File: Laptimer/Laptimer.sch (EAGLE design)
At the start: 64 parts, among them IC1 MCP73831/OT, IC5 NE555D, Q1 8mhz, Q4 PBSS4120T, X1 mini-usb

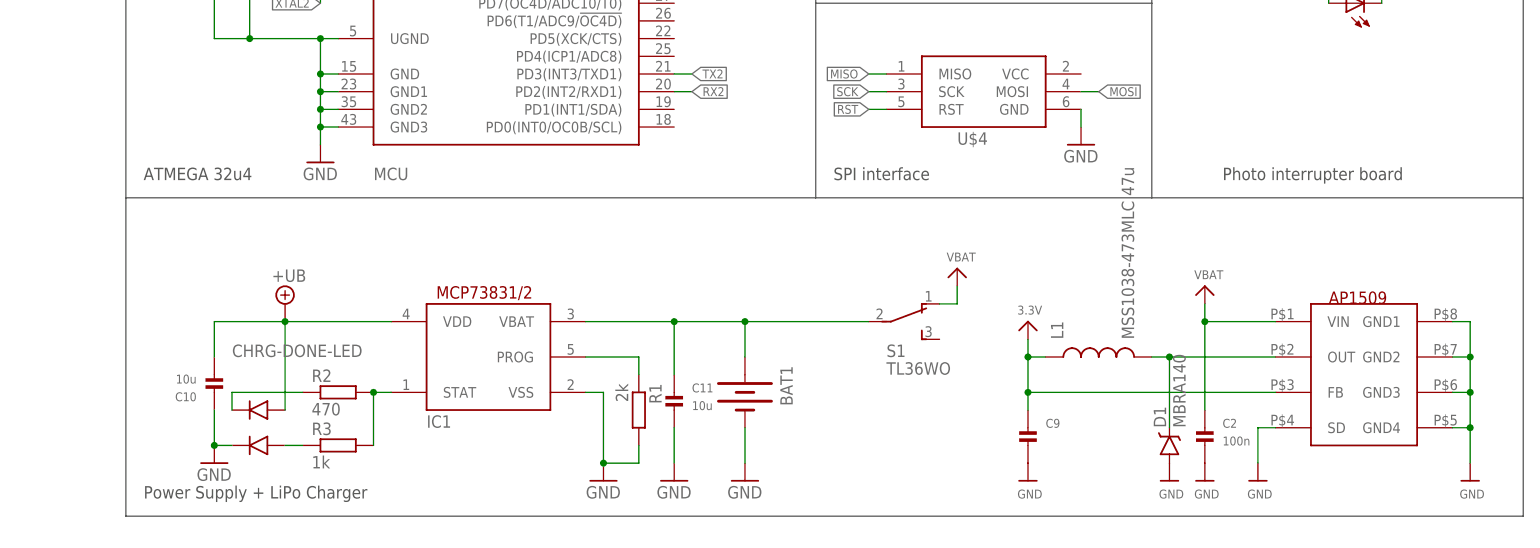
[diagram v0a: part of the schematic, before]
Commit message: power supply update
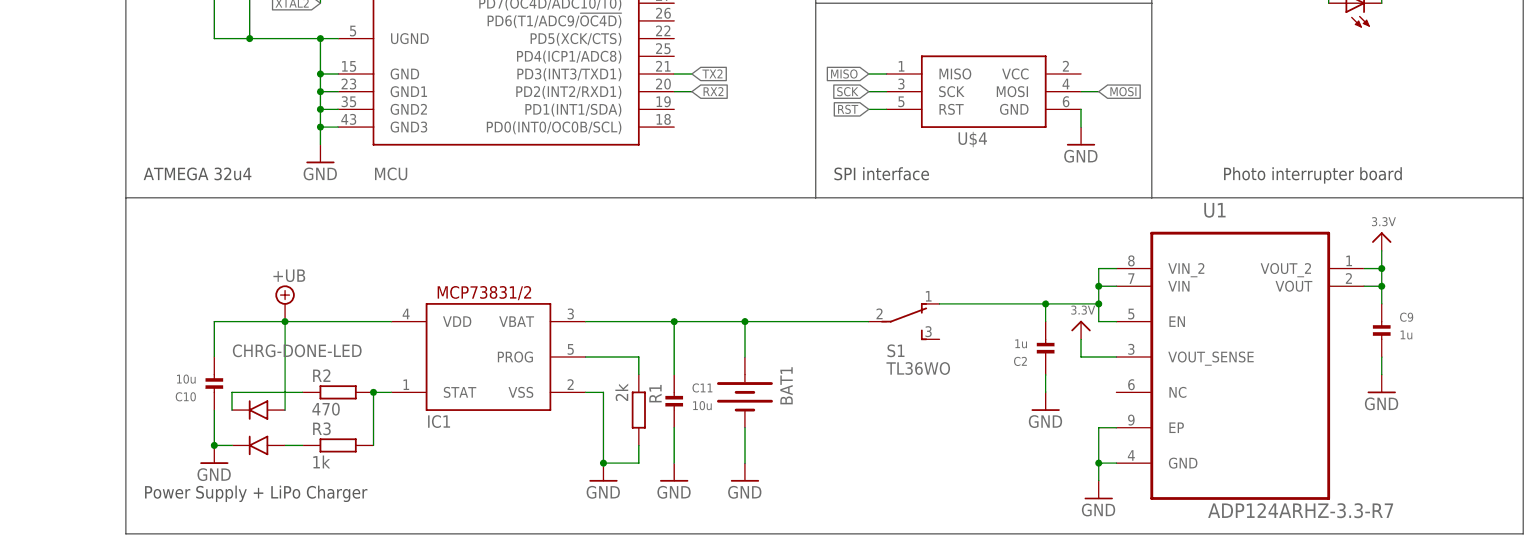
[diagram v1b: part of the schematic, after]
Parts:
- removed D1: MBRA140, SparkFun-DiscreteSemi:MBRA140
- removed L1: MSS1038-473MLC 47u, SparkFun-Passives:INDUCTORPWR
- removed U$2: AP1509, unicorn_v2:AP1509
- added U1: ADP124ARHZ-3.3-R7, Analog Devices_By_element14_Batch_1:ADP124ARHZ-3.3-R7
- C2: value 100n -> 1u; device microbuilder:CAP_CERAMIC_0603MP -> microbuilder:CAP_CERAMIC_0805MP
- C9: value (none) -> 1u
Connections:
- removed net VBAT: C2.P$1, S1.O, U$2.VIN
- net 3.3V: now also U1.VOUT, U1.VOUT_2, U1.VOUT_SENSE; no longer L1.1, U$2.FB
- net GND: now also C2.P$1, U1.EP, U1.GND; no longer C2.P$2, D1.A, U$2.GND1, U$2.GND2, U$2.GND3, U$2.GND4, U$2.SD
- net N$17: now also C2.P$2, S1.O, U1.EN, U1.VIN, U1.VIN_2; no longer D1.C, L1.2, U$2.OUT
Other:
- moved on the sheet: C2, C9
